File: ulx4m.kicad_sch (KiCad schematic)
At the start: 10 parts

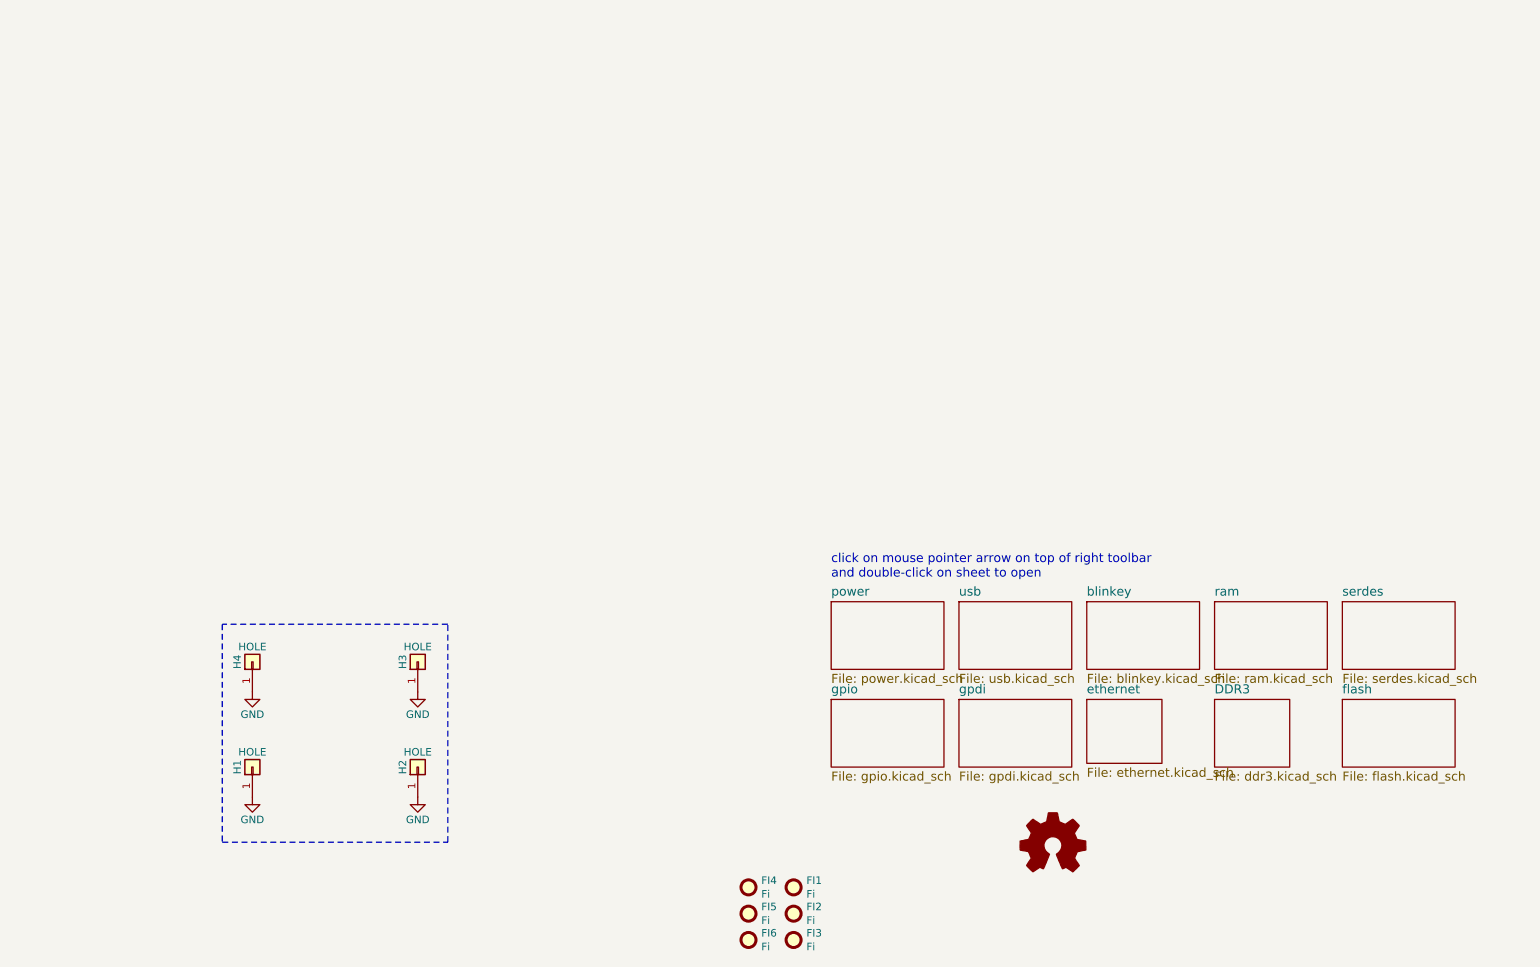
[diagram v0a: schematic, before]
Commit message: Adding schematics
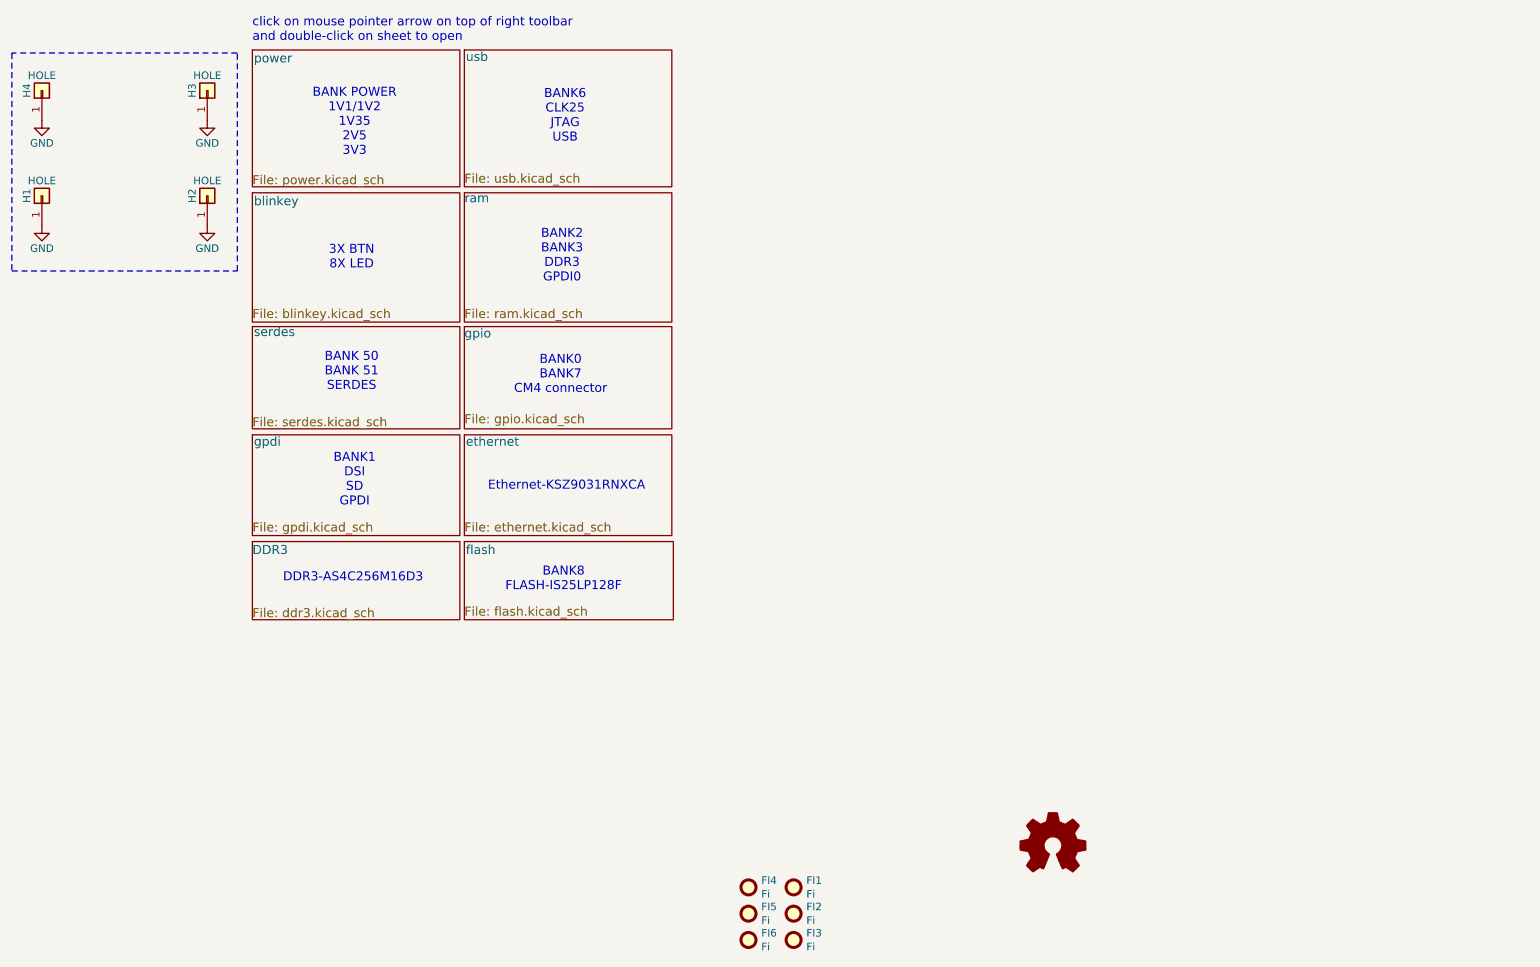
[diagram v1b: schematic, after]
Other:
- note added: "3X BTN 8X LED"
- note added: "BANK 50 BANK 51 SERDES"
- note added: "BANK POWER 1V1/1V2 1V35 2V5 3V3"
- note added: "BANK0 BANK7 CM4 connector"
- note added: "BANK1 DSI SD GPDI"
- note added: "BANK2 BANK3 DDR3 GPDI0"
- note added: "BANK6 CLK25 JTAG USB"
- note added: "BANK8 FLASH-IS25LP128F"
- note added: "DDR3-AS4C256M16D3"
- note added: "Ethernet-KSZ9031RNXCA"
- moved on the sheet: H1, H2, H3, H4
